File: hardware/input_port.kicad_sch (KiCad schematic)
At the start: 1 part, among them J401 10061913-102PLF

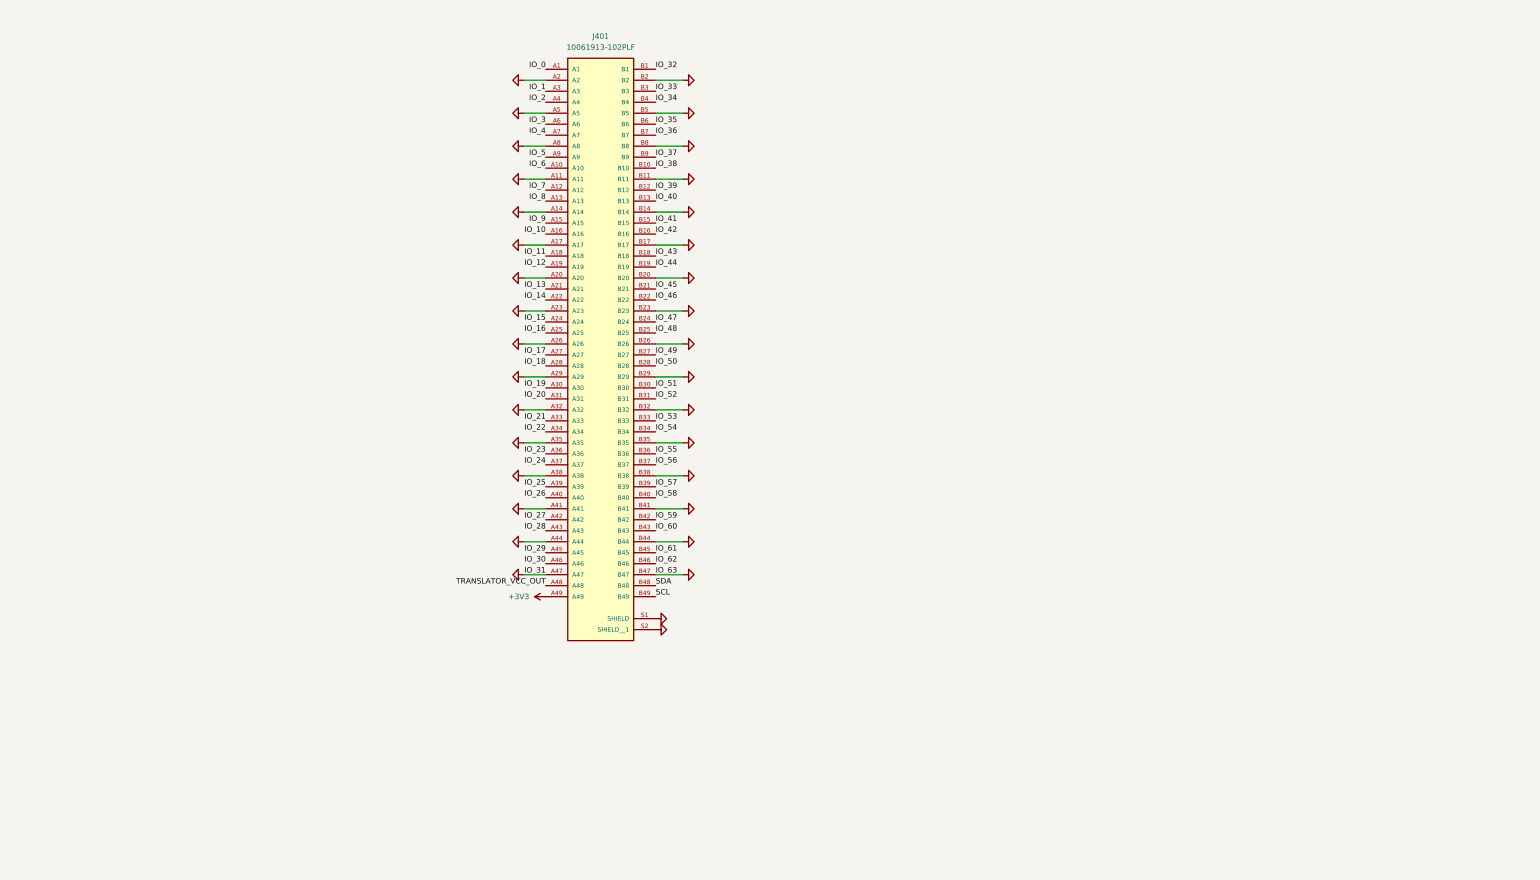
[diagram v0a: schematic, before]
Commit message: Save
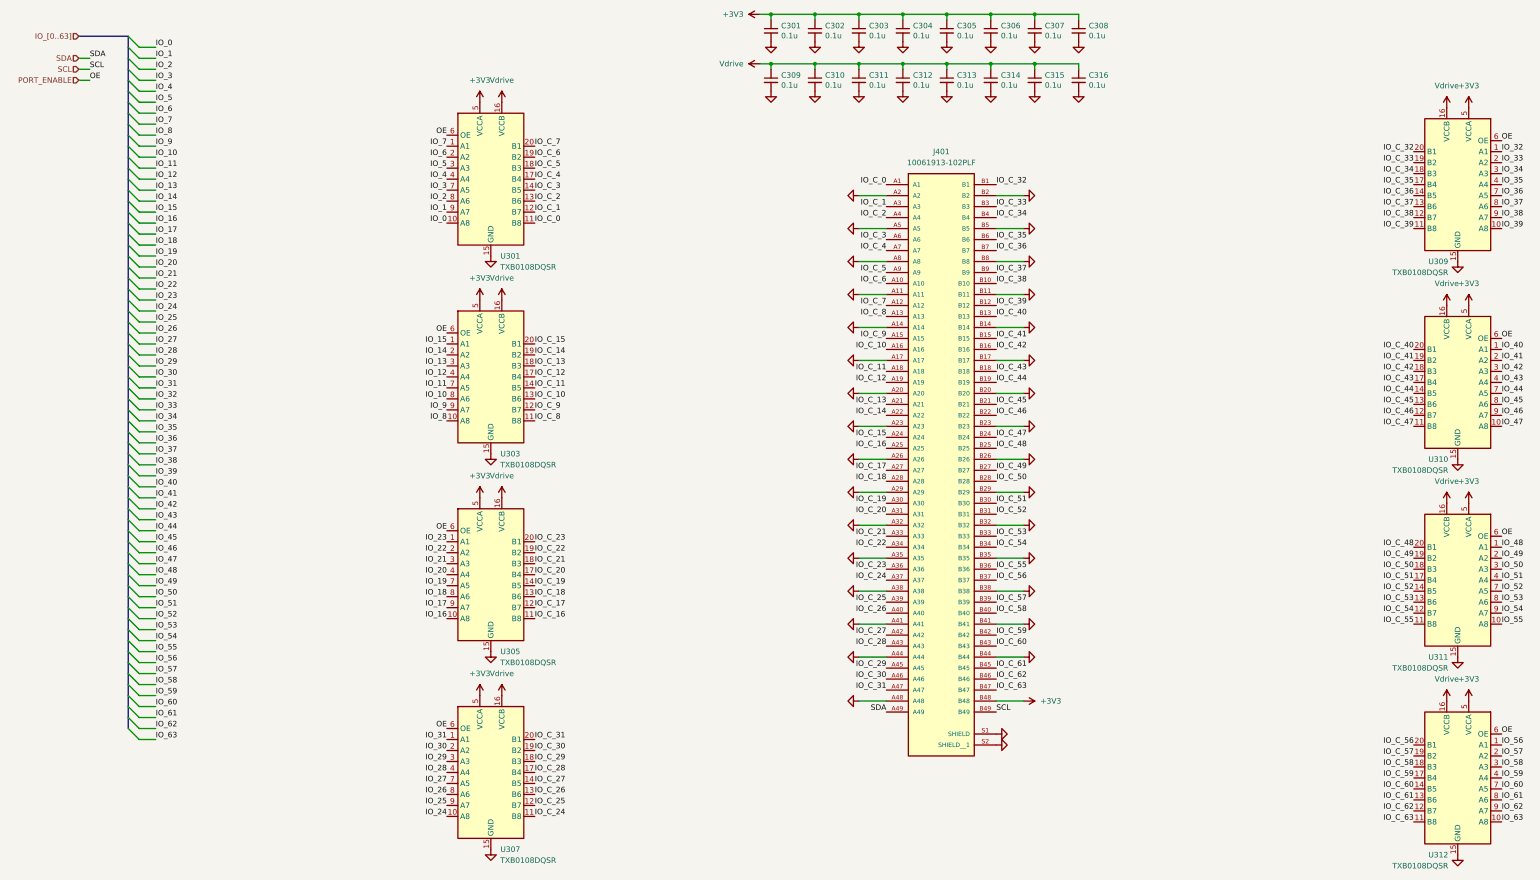
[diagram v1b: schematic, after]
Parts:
- added C301, C302, C303, C304, C305, C306, C307, C308, C309, C310, C311, C312, C313, C314, C315, C316: 0.1u, passive:C_0201, symbol Device:C_Small
- added U301, U303, U305, U307, U309, U310, U311, U312: TXB0108DQSR, Package_SON:USON-20_2x4mm_P0.4mm, symbol Logic_LevelTranslator:TXB0108DQSR
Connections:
- net TRANSLATOR_VCC_OUT is gone; now on net GND: J401.A48
- net +3V3: now also J401.B48, C301.1, C302.1, C303.1, C304.1, C305.1, C306.1, C307.1, C308.1, U301.5 (VCCA), U303.5 (VCCA), U305.5 (VCCA), U307.5 (VCCA), U309.5 (VCCA), U310.5 (VCCA), U311.5 (VCCA), U312.5 (VCCA); no longer J401.A49
- net GND: now also C301.2, C302.2, C303.2, C304.2, C305.2, C306.2, C307.2, C308.2, C309.2, C310.2, C311.2, C312.2, C313.2, C314.2, C315.2, C316.2, U301.15 (GND), U303.15 (GND), U305.15 (GND), U307.15 (GND), U309.15 (GND), U310.15 (GND), U311.15 (GND), U312.15 (GND); no longer J401.A47, J401.B47
- net IO_0: now also U301.10 (A8); no longer J401.A1
- net IO_1: now also U301.9 (A7); no longer J401.A3
- net IO_10: now also U303.8 (A6); no longer J401.A16
- net IO_11: now also U303.7 (A5); no longer J401.A18
- net IO_12: now also U303.4 (A4); no longer J401.A19
- net IO_13: now also U303.3 (A3); no longer J401.A21
- net IO_14: now also U303.2 (A2); no longer J401.A22
- net IO_15: now also U303.1 (A1); no longer J401.A24
- net IO_16: now also U305.10 (A8); no longer J401.A25
- net IO_17: now also U305.9 (A7); no longer J401.A27
- net IO_18: now also U305.8 (A6); no longer J401.A28
- net IO_19: now also U305.7 (A5); no longer J401.A30
- net IO_2: now also U301.8 (A6); no longer J401.A4
- net IO_20: now also U305.4 (A4); no longer J401.A31
- net IO_21: now also U305.3 (A3); no longer J401.A33
- net IO_22: now also U305.2 (A2); no longer J401.A34
- net IO_23: now also U305.1 (A1); no longer J401.A36
- net IO_24: now also U307.10 (A8); no longer J401.A37
- net IO_25: now also U307.9 (A7); no longer J401.A39
- net IO_26: now also U307.8 (A6); no longer J401.A40
- net IO_27: now also U307.7 (A5); no longer J401.A42
- net IO_28: now also U307.4 (A4); no longer J401.A43
- net IO_29: now also U307.3 (A3); no longer J401.A45
- net IO_3: now also U301.7 (A5); no longer J401.A6
- net IO_30: now also U307.2 (A2); no longer J401.A46
- net IO_32: now also U309.1 (A1); no longer J401.B1
- net IO_33: now also U309.2 (A2); no longer J401.B3
- net IO_34: now also U309.3 (A3); no longer J401.B4
- net IO_35: now also U309.4 (A4); no longer J401.B6
- net IO_36: now also U309.7 (A5); no longer J401.B7
- net IO_37: now also U309.8 (A6); no longer J401.B9
- net IO_38: now also U309.9 (A7); no longer J401.B10
- net IO_39: now also U309.10 (A8); no longer J401.B12
- net IO_4: now also U301.4 (A4); no longer J401.A7
- net IO_40: now also U310.1 (A1); no longer J401.B13
- net IO_41: now also U310.2 (A2); no longer J401.B15
- net IO_42: now also U310.3 (A3); no longer J401.B16
- net IO_43: now also U310.4 (A4); no longer J401.B18
- net IO_44: now also U310.7 (A5); no longer J401.B19
- net IO_45: now also U310.8 (A6); no longer J401.B21
- net IO_46: now also U310.9 (A7); no longer J401.B22
- net IO_47: now also U310.10 (A8); no longer J401.B24
- net IO_48: now also U311.1 (A1); no longer J401.B25
- net IO_49: now also U311.2 (A2); no longer J401.B27
- net IO_5: now also U301.3 (A3); no longer J401.A9
- net IO_50: now also U311.3 (A3); no longer J401.B28
- net IO_51: now also U311.4 (A4); no longer J401.B30
- net IO_52: now also U311.7 (A5); no longer J401.B31
- net IO_53: now also U311.8 (A6); no longer J401.B33
- net IO_54: now also U311.9 (A7); no longer J401.B34
- net IO_55: now also U311.10 (A8); no longer J401.B36
- net IO_56: now also U312.1 (A1); no longer J401.B37
- net IO_57: now also U312.2 (A2); no longer J401.B39
- net IO_58: now also U312.3 (A3); no longer J401.B40
- net IO_59: now also U312.4 (A4); no longer J401.B42
- net IO_6: now also U301.2 (A2); no longer J401.A10
- net IO_60: now also U312.7 (A5); no longer J401.B43
- net IO_61: now also U312.8 (A6); no longer J401.B45
- net IO_62: now also U312.9 (A7); no longer J401.B46
- net IO_7: now also U301.1 (A1); no longer J401.A12
- net IO_8: now also U303.10 (A8); no longer J401.A13
- net IO_9: now also U303.9 (A7); no longer J401.A15
- net SDA: now also J401.A49; no longer J401.B48
- new net IO_31: U307.1 (A1)
- new net IO_63: U312.10 (A8)
- new net IO_C_0: J401.A1, U301.11 (B8)
- new net IO_C_1: J401.A3, U301.12 (B7)
- new net IO_C_10: J401.A16, U303.13 (B6)
- new net IO_C_11: J401.A18, U303.14 (B5)
- new net IO_C_12: J401.A19, U303.17 (B4)
- new net IO_C_13: J401.A21, U303.18 (B3)
- new net IO_C_14: J401.A22, U303.19 (B2)
- new net IO_C_15: J401.A24, U303.20 (B1)
- new net IO_C_16: J401.A25, U305.11 (B8)
- new net IO_C_17: J401.A27, U305.12 (B7)
- new net IO_C_18: J401.A28, U305.13 (B6)
- new net IO_C_19: J401.A30, U305.14 (B5)
- new net IO_C_2: J401.A4, U301.13 (B6)
- new net IO_C_20: J401.A31, U305.17 (B4)
- new net IO_C_21: J401.A33, U305.18 (B3)
- new net IO_C_22: J401.A34, U305.19 (B2)
- new net IO_C_23: J401.A36, U305.20 (B1)
- new net IO_C_24: J401.A37, U307.11 (B8)
- new net IO_C_25: J401.A39, U307.12 (B7)
- new net IO_C_26: J401.A40, U307.13 (B6)
- new net IO_C_27: J401.A42, U307.14 (B5)
- new net IO_C_28: J401.A43, U307.17 (B4)
- new net IO_C_29: J401.A45, U307.18 (B3)
- new net IO_C_3: J401.A6, U301.14 (B5)
- new net IO_C_30: J401.A46, U307.19 (B2)
- new net IO_C_31: J401.A47, U307.20 (B1)
- new net IO_C_32: J401.B1, U309.20 (B1)
- new net IO_C_33: J401.B3, U309.19 (B2)
- new net IO_C_34: J401.B4, U309.18 (B3)
- new net IO_C_35: J401.B6, U309.17 (B4)
- new net IO_C_36: J401.B7, U309.14 (B5)
- new net IO_C_37: J401.B9, U309.13 (B6)
- new net IO_C_38: J401.B10, U309.12 (B7)
- new net IO_C_39: J401.B12, U309.11 (B8)
- new net IO_C_4: J401.A7, U301.17 (B4)
- new net IO_C_40: J401.B13, U310.20 (B1)
- new net IO_C_41: J401.B15, U310.19 (B2)
- new net IO_C_42: J401.B16, U310.18 (B3)
- new net IO_C_43: J401.B18, U310.17 (B4)
- new net IO_C_44: J401.B19, U310.14 (B5)
- new net IO_C_45: J401.B21, U310.13 (B6)
- new net IO_C_46: J401.B22, U310.12 (B7)
- new net IO_C_47: J401.B24, U310.11 (B8)
- new net IO_C_48: J401.B25, U311.20 (B1)
- new net IO_C_49: J401.B27, U311.19 (B2)
- new net IO_C_5: J401.A9, U301.18 (B3)
- new net IO_C_50: J401.B28, U311.18 (B3)
- new net IO_C_51: J401.B30, U311.17 (B4)
- new net IO_C_52: J401.B31, U311.14 (B5)
- new net IO_C_53: J401.B33, U311.13 (B6)
- new net IO_C_54: J401.B34, U311.12 (B7)
- new net IO_C_55: J401.B36, U311.11 (B8)
- new net IO_C_56: J401.B37, U312.20 (B1)
- new net IO_C_57: J401.B39, U312.19 (B2)
- new net IO_C_58: J401.B40, U312.18 (B3)
- new net IO_C_59: J401.B42, U312.17 (B4)
- new net IO_C_6: J401.A10, U301.19 (B2)
- new net IO_C_60: J401.B43, U312.14 (B5)
- new net IO_C_61: J401.B45, U312.13 (B6)
- new net IO_C_62: J401.B46, U312.12 (B7)
- new net IO_C_63: J401.B47, U312.11 (B8)
- new net IO_C_7: J401.A12, U301.20 (B1)
- new net IO_C_8: J401.A13, U303.11 (B8)
- new net IO_C_9: J401.A15, U303.12 (B7)
- new net PORT_ENABLE: U301.6 (OE), U303.6 (OE), U305.6 (OE), U307.6 (OE), U309.6 (OE), U310.6 (OE), U311.6 (OE), U312.6 (OE)
- new net Vdrive: C309.1, C310.1, C311.1, C312.1, C313.1, C314.1, C315.1, C316.1, U301.16 (VCCB), U303.16 (VCCB), U305.16 (VCCB), U307.16 (VCCB), U309.16 (VCCB), U310.16 (VCCB), U311.16 (VCCB), U312.16 (VCCB)
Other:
- moved on the sheet: J401
